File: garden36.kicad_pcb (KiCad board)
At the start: 2 copper layers, 41 parts, among them J1 Conn_01x02, SW1 SW_SPDT, SW2 SW_Push, U1 nice_nano

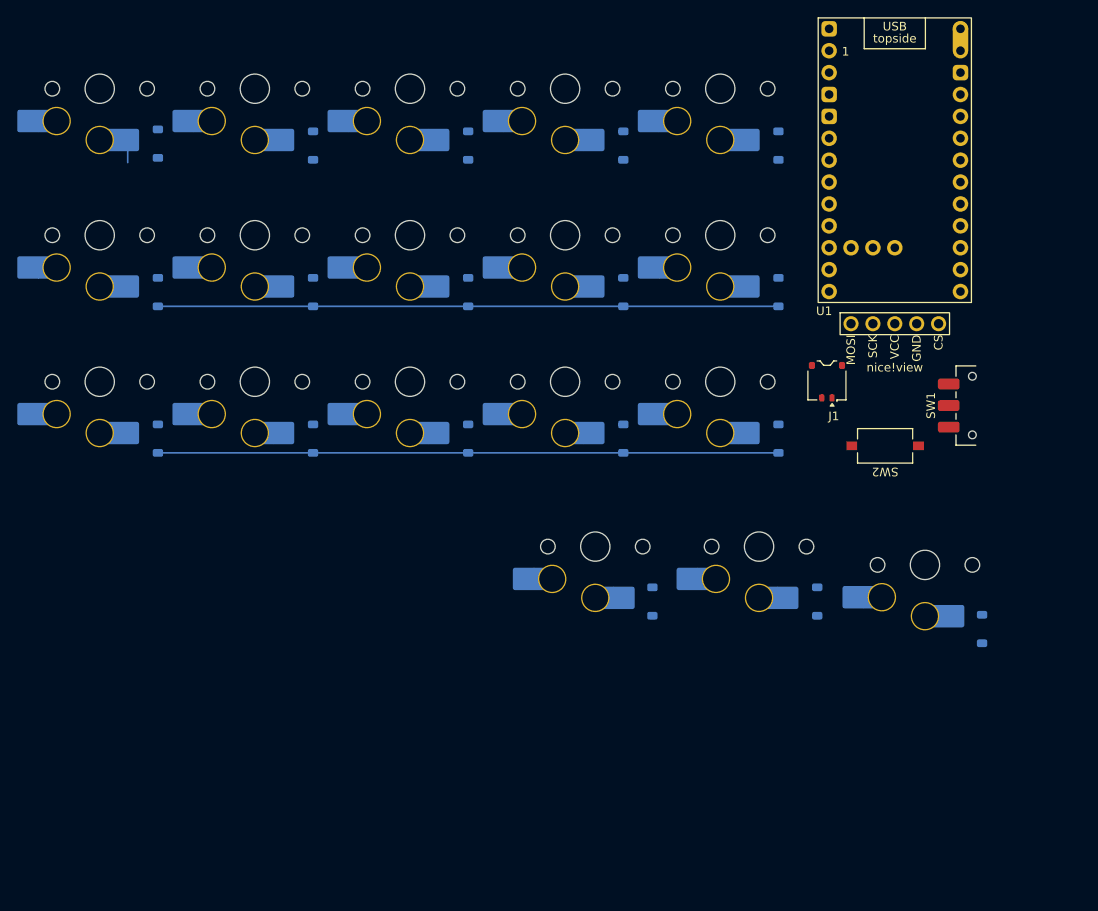
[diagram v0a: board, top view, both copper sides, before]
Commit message: Finished basic layout without any routing
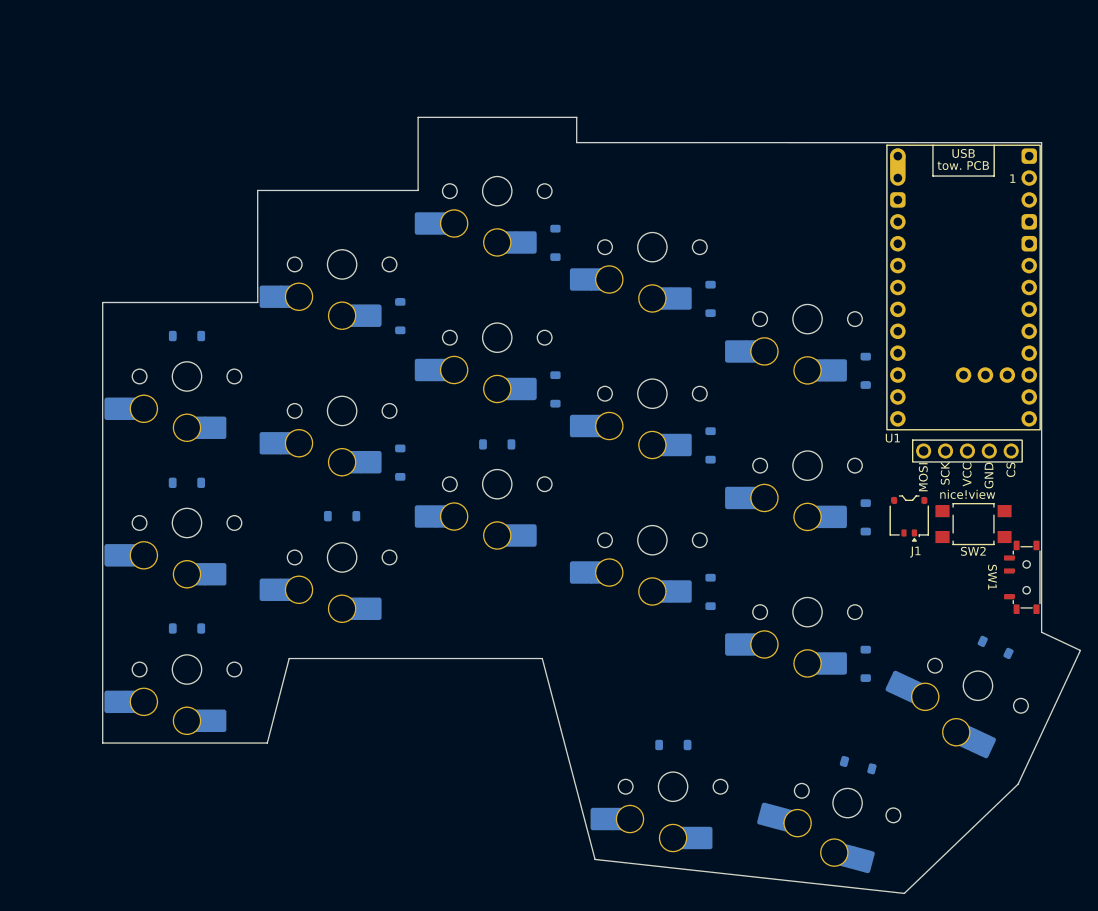
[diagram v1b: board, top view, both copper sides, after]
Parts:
- SW1: footprint Button_Switch_SMD:SW_SPDT_CK_JS102011SAQN -> PCM_marbastlib-various:SW_MSK12C02-HB
- SW2: footprint Button_Switch_SMD:SW_Tactile_SPST_NO_Straight_CK_PTS636Sx25SMTRLFS -> Button_Switch_SMD:SW_SPST_TL3305A
- U1: footprint PCM_marbastlib-xp-promicroish:nice_nano_AH_USBup -> PCM_marbastlib-xp-promicroish:nice_nano_AH_USBdn
- moved CH11 34.9 mm to (40.5, 112.9)
- moved CH1 34.9 mm to (40.5, 78.9)
- moved CH6 34.9 mm to (40.5, 95.9)
- moved CH17 31.5 mm to (117.1, 128.4), turned to 165 degrees
- moved CH16 29.3 mm to (96.9, 126.5)
- moved CH15 28.6 mm to (112.5, 106.2)
- moved CH10 28.6 mm to (112.5, 89.2)
- moved CH5 28.6 mm to (112.5, 72.2)
- moved D10 28.0 mm to (119.2, 95.2)
- moved D15 28.0 mm to (119.2, 112.2)
- moved D5 28.0 mm to (119.2, 78.2)
- moved CH12 22.8 mm to (58.5, 99.9)
- moved CH2 22.8 mm to (58.5, 65.9)
- moved CH7 22.8 mm to (58.5, 82.9)
- moved D1 22.6 mm to (40.5, 74.2), turned to 0 degrees
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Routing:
- net ROW2: track 72.0 -> 0.00 mm
- net ROW1: track 72.0 -> 0.00 mm
- net Net-(D1-A): track 2.62 -> 0.00 mm
- net Net-(D5-A): track 1.70 -> 0.00 mm
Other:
- board outline added: 113.4 x 90 mm
- rule pad_to_mask_clearance: 0 -> 0.038
